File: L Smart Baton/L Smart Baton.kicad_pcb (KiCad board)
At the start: 2 copper layers, 25 x 200 mm, 51 parts, among them J1 USB4105-GF-A, SW1 B3U-1000P, SW1_R1 1k, U1 MDBT50Q-1MV2, U2 LSM6DSOX, U3 BQ24074RGT, U4 TPS63001

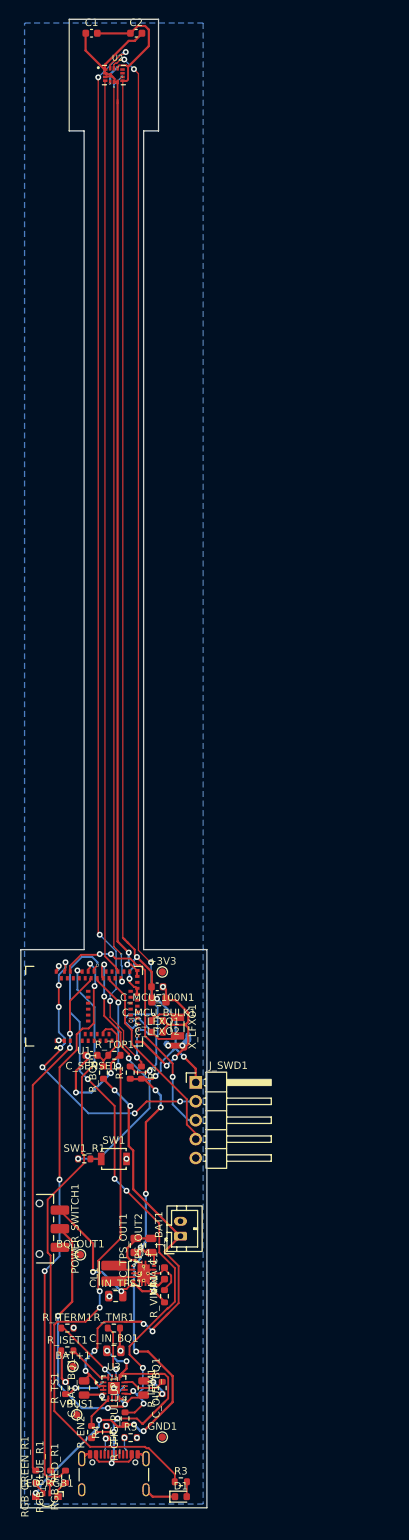
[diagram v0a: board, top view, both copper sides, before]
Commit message: ALMOST FINAL
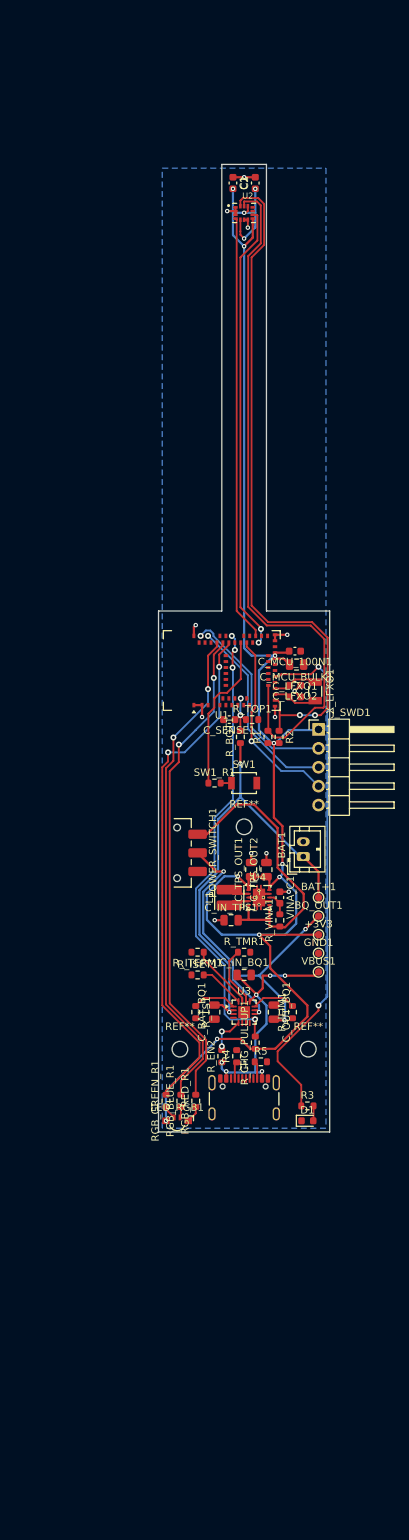
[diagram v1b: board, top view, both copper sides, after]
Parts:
- added REF**: MountingHole_2.1mm, MountingHole:MountingHole_2.1mm, F.Cu at (210.0, 148.5)
- added REF**: MountingHole_2.1mm, MountingHole:MountingHole_2.1mm, F.Cu at (218.6, 178.4)
- added REF**: MountingHole_2.1mm, MountingHole:MountingHole_2.1mm, F.Cu at (201.4, 178.4)
- moved BAT+1 71.1 mm to (220.0, 158.0)
- moved GND1 68.3 mm to (220.0, 165.5)
- moved VBUS1 67.8 mm to (220.0, 168.0)
- moved BQ_OUT1 55.6 mm to (220.0, 160.5)
- moved POWER_SWITCH1 53.8 mm to (201.0, 152.0)
- moved J_BAT1 53.6 mm to (217.9, 152.5)
- moved C_BAT_BQ1 53.4 mm to (206.0, 173.4)
- moved C_IN_BQ1 53.4 mm to (210.0, 168.4)
- moved C_OUT_BQ1 53.4 mm to (214.0, 173.4)
- moved J1 53.4 mm to (210.0, 186.0)
- moved LED_RGB1 53.4 mm to (201.0, 188.0)
- moved R4 53.4 mm to (209.0, 179.3)
- moved R5 53.4 mm to (212.2, 180.1)
- moved RGB_BLUE_R1 53.4 mm to (201.5, 185.3)
- moved RGB_GREEN_R1 53.4 mm to (199.5, 185.3)
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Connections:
- U1 pad 22: unconnected-(U1-P0.06-Pad22) -> /BLE_LED
- U1 pad 43: /BLE_LED -> unconnected-(U1-P0.21-Pad43)
- U1 pad 46: /RGB_RED -> unconnected-(U1-P0.22-Pad46)
- U1 pad 47: unconnected-(U1-P1.00-Pad47) -> /RGB_RED
- U1 pad 48: /RGB_BLUE -> unconnected-(U1-P0.24-Pad48)
- U1 pad 49: unconnected-(U1-P0.25-Pad49) -> /RGB_BLUE
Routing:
- net GND: track 225.6 -> 26.1 mm, vias 25 -> 12
- net /IMU_INT1: track 120.4 -> 57.2 mm
- net /IMU_INT2: track 122.7 -> 60.3 mm, vias 4 -> 2
- net Net-(U1-P0.27): track 146.7 -> 92.2 mm, vias 6 -> 2
- net Net-(U1-P0.26): track 147.9 -> 94.8 mm, vias 5 -> 0
- net +3V3: track 254.7 -> 221.6 mm, vias 17 -> 13
- net /CHG_STATUS: track 79.1 -> 62.0 mm, vias 7 -> 4
- net Net-(POWER_SWITCH1-A): track 23.7 -> 40.5 mm, vias 4 -> 0
- net /BLE_LED: track 86.0 -> 70.0 mm, vias 4 -> 2
- net /USER_BTN: track 36.0 -> 21.2 mm, vias 4 -> 0
- net /SWDCLK: track 40.6 -> 27.1 mm, vias 7 -> 1
- net /SW_POW: track 39.8 -> 52.1 mm
- net /RGB_RED: track 76.1 -> 66.5 mm, vias 4 -> 2
- net /SWDIO: track 35.4 -> 26.4 mm, vias 3 -> 1
- net Net-(U3-IN): track 40.6 -> 35.3 mm, vias 5 -> 6
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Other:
- board size 25 x 200 mm -> 23 x 130 mm
